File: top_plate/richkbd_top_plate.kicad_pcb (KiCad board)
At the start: 2 copper layers, 125.8 x 119 mm, 25 parts, among them K0 key-diode-led, K1 key-diode-led, K10 key-diode-led, K11 key-diode-led, K12 key-diode-led, K2 key-diode-led, K20 key-diode-led, K21 key-diode-led, K22 key-diode-led, K30 key-diode-led, K31 key-diode-led, K32 key-diode-led, K33 key-diode-led, K40 key-diode-led, K41 key-diode-led, K42 key-diode-led, K43 key-diode-led, K50 key-diode-led, K51 key-diode-led, K52 key-diode-led, K53 key-diode-led

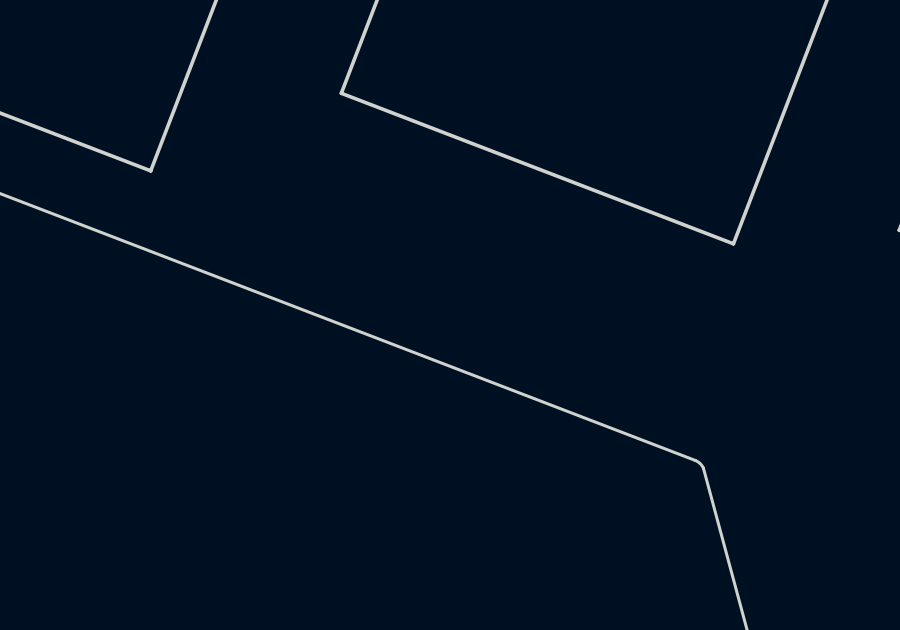
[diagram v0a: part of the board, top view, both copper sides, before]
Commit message: A good start at the documentation.
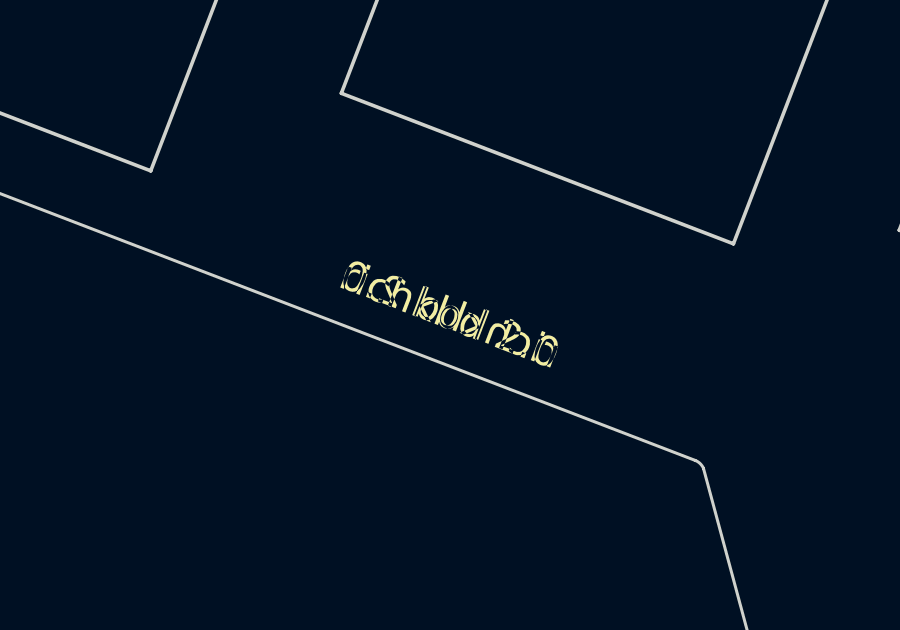
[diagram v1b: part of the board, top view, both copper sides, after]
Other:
- board text added: "richkbd 2.0"
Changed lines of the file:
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@@
   (gr_line (start 159.887965 70.150621) (end 158.131936 74.725228) (layer "F.Fab") (width 0.1))
   (gr_line (start 156.722691 71.559894) (end 161.297233 73.315896) (layer "F.Fab") (width 0.1))
+  (gr_text "richkbd 2.0" (at 99.68 92.07 -21) (layer "F.SilkS")
+    (effects (font (size 1 1) (thickness 0.15)) (justify mirror))
+  )
+  (gr_text "richkbd 2.0" (at 99.66 92.08 -21) (layer "F.SilkS")
+    (effects (font (size 1 1) (thickness 0.15)))
+  )
 )
